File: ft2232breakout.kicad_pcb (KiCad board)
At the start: 2 copper layers, 43.2 x 35.6 mm, 24 parts, among them J1 USB_B_Micro, J2 Conn_01x20, J3 Conn_01x20, U1 FT2232H, U2 NCP1117-3.3_SOT223, U3 93CxxA

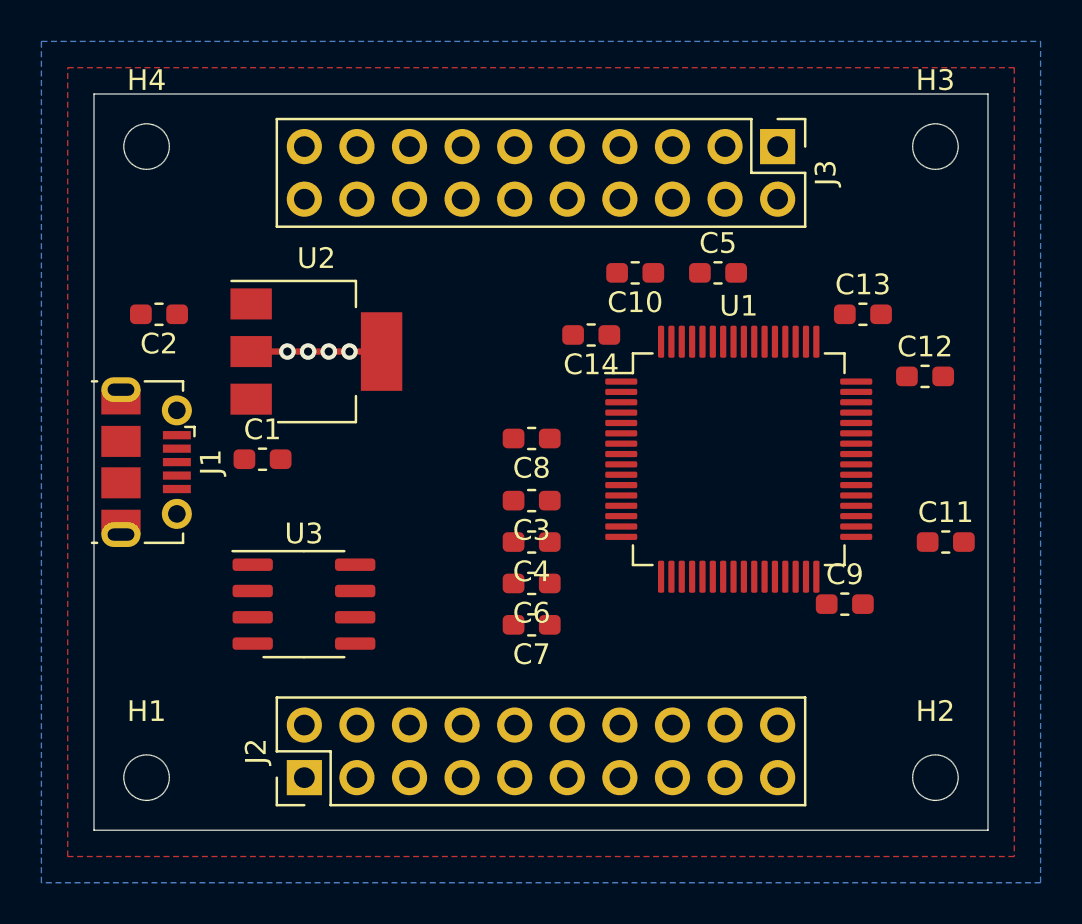
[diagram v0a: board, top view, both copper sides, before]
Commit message: Nearly there
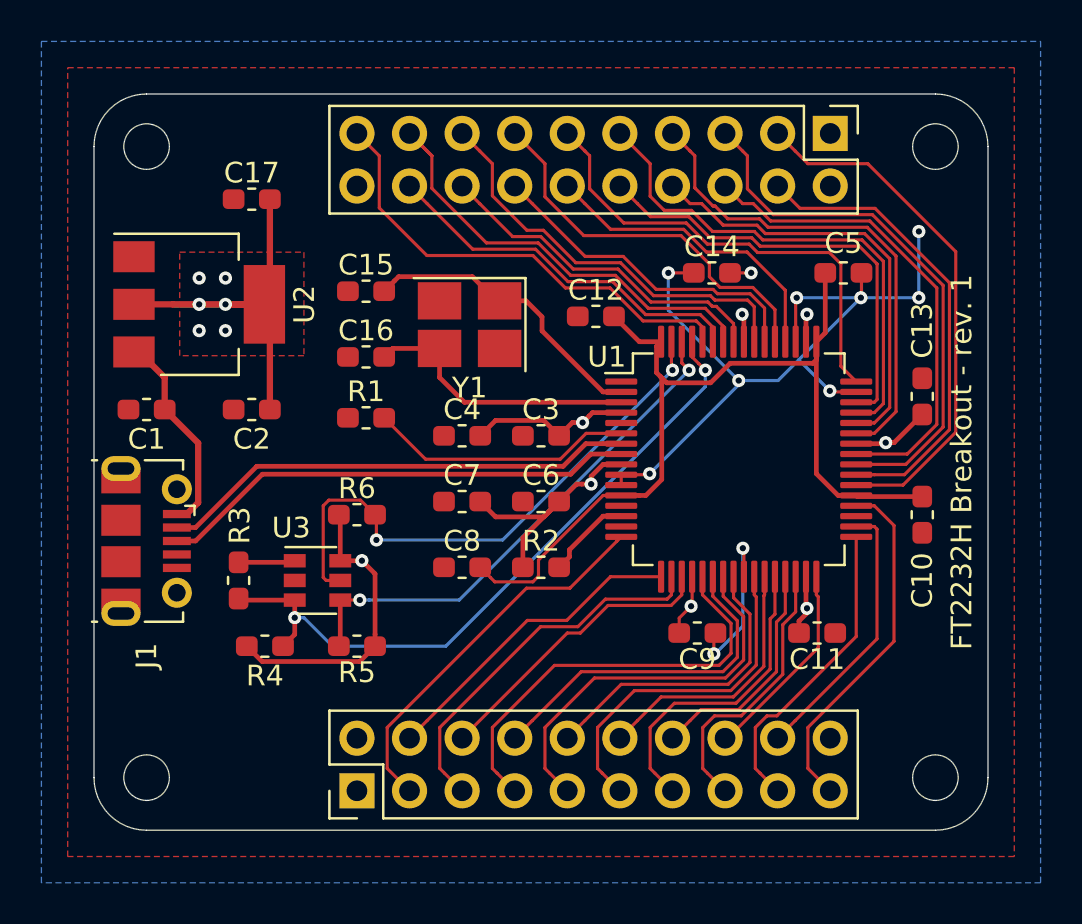
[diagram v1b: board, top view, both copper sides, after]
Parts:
- added C15: 27pF, Capacitor_SMD:C_0603_1608Metric_Pad1.05x0.95mm_HandSolder, F.Cu at (163.0, 95.9)
- added C16: 27pF, Capacitor_SMD:C_0603_1608Metric_Pad1.05x0.95mm_HandSolder, F.Cu at (163.0, 99.1)
- added C17: 4.7uF, Capacitor_SMD:C_0603_1608Metric_Pad1.05x0.95mm_HandSolder, F.Cu at (157.5, 91.4)
- added R1: 12k, Resistor_SMD:R_0603_1608Metric_Pad1.05x0.95mm_HandSolder, F.Cu at (163.0, 102.0)
- added R2: 1k, Resistor_SMD:R_0603_1608Metric_Pad1.05x0.95mm_HandSolder, F.Cu at (171.4, 109.2)
- added R3: 2.2k, Resistor_SMD:R_0603_1608Metric_Pad1.05x0.95mm_HandSolder, F.Cu at (156.8, 109.9)
- added R4: 10k, Resistor_SMD:R_0603_1608Metric_Pad1.05x0.95mm_HandSolder, F.Cu at (158.1, 113.0)
- added R5: 10k, Resistor_SMD:R_0603_1608Metric_Pad1.05x0.95mm_HandSolder, F.Cu at (162.6, 113.0)
- added R6: 10k, Resistor_SMD:R_0603_1608Metric_Pad1.05x0.95mm_HandSolder, F.Cu at (162.6, 106.7)
- added Y1: 12MHz, Crystal:Crystal_SMD_3225-4Pin_3.2x2.5mm_HandSoldering, F.Cu at (168.0, 97.5)
- U3: value 93CxxA -> 93LCxxAxxOT; footprint Package_SO:SOIC-8_3.9x4.9mm_P1.27mm -> Package_TO_SOT_SMD:SOT-23-6
- moved C10 18.1 mm to (189.9, 106.7), turned to 270 degrees
- moved C12 16.2 mm to (174.1, 97.1), turned to 180 degrees
- moved C11 7.61 mm to (184.8, 112.4)
- moved C9 7.26 mm to (179.0, 112.4)
- moved C8 7.07 mm to (167.6, 109.2)
- moved C7 6.84 mm to (167.6, 106.0)
- moved C14 6.56 mm to (179.7, 95.0)
- moved C2 6.42 mm to (157.5, 101.6)
- moved C4 6.13 mm to (167.6, 102.9)
- moved U2 6.10 mm to (154.9, 96.5)
- moved C1 6.09 mm to (152.4, 101.6), turned to 180 degrees
- moved C5 6.06 mm to (186.1, 95.0)
- moved C13 4.89 mm to (189.9, 101.0), turned to 90 degrees
- moved C6 3.98 mm to (171.4, 106.0)
- moved J1 3.81 mm to (152.4, 108.0)
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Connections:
- net Net-(J2-Pad10) renamed /AD7
- net Net-(J2-Pad11) renamed /AC0
- net Net-(J2-Pad12) renamed /AC1
- net Net-(J2-Pad13) renamed /AC2
- net Net-(J2-Pad14) renamed /AC3
- net Net-(J2-Pad15) renamed /AC4
- net Net-(J2-Pad16) renamed /AC5
- net Net-(J2-Pad17) renamed /AC6
- net Net-(J2-Pad18) renamed /AC7
- net Net-(J2-Pad3) renamed /AD0
- net Net-(J2-Pad4) renamed /AD1
- net Net-(J2-Pad5) renamed /AD2
- net Net-(J2-Pad6) renamed /AD3
- net Net-(J2-Pad7) renamed /AD4
- net Net-(J2-Pad8) renamed /AD5
- net Net-(J2-Pad9) renamed /AD6
- net Net-(J3-Pad10) renamed /BD7
- net Net-(J3-Pad11) renamed /BC0
- net Net-(J3-Pad12) renamed /BC1
- net Net-(J3-Pad13) renamed /BC2
- net Net-(J3-Pad14) renamed /BC3
- net Net-(J3-Pad15) renamed /BC4
- net Net-(J3-Pad16) renamed /BC5
- net Net-(J3-Pad17) renamed /BC6
- net Net-(J3-Pad18) renamed /BC7
- net Net-(J3-Pad3) renamed /BD0
- net Net-(J3-Pad4) renamed /BD1
- net Net-(J3-Pad5) renamed /BD2
- net Net-(J3-Pad6) renamed /BD3
- net Net-(J3-Pad7) renamed /BD4
- net Net-(J3-Pad8) renamed /BD5
- net Net-(J3-Pad9) renamed /BD6
- J2 pad 1: Net-(J2-Pad1) -> +3V3
- J2 pad 19: Net-(J2-Pad19) -> /~SUSPEND
- J2 pad 2: Net-(J2-Pad2) -> GND
- J2 pad 20: Net-(J2-Pad20) -> GND
- J3 pad 1: Net-(J3-Pad1) -> +3V3
- J3 pad 19: Net-(J3-Pad19) -> /~PWREN
- J3 pad 2: Net-(J3-Pad2) -> GND
- J3 pad 20: Net-(J3-Pad20) -> GND
- U1 pad 1: Net-(U1-Pad1) -> GND
- U1 pad 10: Net-(U1-Pad10) -> GND
- U1 pad 11: Net-(U1-Pad11) -> GND
- U1 pad 13: Net-(U1-Pad13) -> GND
- U1 pad 15: Net-(U1-Pad15) -> GND
- U1 pad 25: Net-(U1-Pad25) -> GND
- U1 pad 35: Net-(U1-Pad35) -> GND
- U1 pad 36: Net-(U1-Pad36) -> /~SUSPEND
- U1 pad 47: Net-(U1-Pad47) -> GND
- U1 pad 5: Net-(U1-Pad5) -> GND
- U1 pad 51: Net-(U1-Pad51) -> GND
- U1 pad 60: Net-(U1-Pad60) -> /~PWREN
- U1 pad 61: Net-(U1-Pad61) -> Net-(R3-Pad2)
- U1 pad 62: Net-(U1-Pad62) -> Net-(R5-Pad1)
- U1 pad 63: Net-(U1-Pad63) -> Net-(R6-Pad1)
- U3 pad 2: Net-(U3-Pad2) -> GND
- U3 pad 3: Net-(U3-Pad3) -> Net-(R3-Pad2)
- U3 pad 4: Net-(U3-Pad4) -> Net-(R5-Pad1)
- U3 pad 5: Net-(U3-Pad5) -> Net-(R6-Pad1)
- U3 pad 6: Net-(U3-Pad6) -> +3V3
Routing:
- net +3V3: track 6.30 -> 69.2 mm, vias 4 -> 15
- net GND: track 0.00 -> 47.6 mm, vias 0 -> 10
- net +1V8: track 0.00 -> 45.6 mm
- net Net-(R3-Pad2): track 0.00 -> 33.2 mm, vias 0 -> 2
- net Net-(R6-Pad1): track 0.00 -> 27.6 mm, vias 0 -> 2
- net /BD2: track 0.00 -> 26.3 mm
- net /BD0: track 0.00 -> 25.6 mm
- net Net-(R5-Pad1): track 0.00 -> 25.2 mm, vias 0 -> 2
- net /BD6: track 0.00 -> 24.6 mm
- net /BD4: track 0.00 -> 24.0 mm
- net /BD3: track 0.00 -> 23.3 mm
- net Net-(J1-Pad3): track 0.00 -> 23.2 mm
- net Net-(J1-Pad2): track 0.00 -> 23.1 mm
- net /BC0: track 0.00 -> 22.7 mm
- net /~PWREN: track 0.00 -> 22.7 mm
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- added copper zone on F.Cu, net +3V3
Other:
- outline, holes or cut-outs redrawn
- net class Default: via_dia 0.8 -> 0.635; via_drill 0.4 -> 0.3
- rule pad_to_mask_clearance: 0.051 -> 0.0508
- board text added: "+3V3 GND"
- board text added: "AC0 AC1"
- board text added: "AC2 AC3"
- board text added: "AC4 AC5"
- board text added: "AC6 AC7"
- board text added: "AD0 AD1"
- board text added: "AD2 AD3"
- board text added: "AD4 AD5"
- board text added: "AD6 AD7"
- board text added: "BC1 BC0"
- board text added: "BC3 BC2"
- board text added: "BC5 BC4"
- board text added: "BC7 BC6"
- board text added: "BD1 BD0"
- board text added: "BD3 BD2"
- board text added: "BD5 BD4"
- board text added: "BD7 BD6"
- board text added: "FT2232H Breakout - rev. 1"
- board text added: "GND +3V3"
- board text added: "GND ~PWREN~"
- board text added: "~SUSPEND~ GND"
